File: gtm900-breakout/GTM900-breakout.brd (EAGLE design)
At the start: 70 x 70 mm, 110 parts, among them IC1 NCP303, IC2 CP2102N_28, J1 AUDIO-JACK3, K1 PJ-002BH-SMT-TR, T2 BC847, T3 BC847, U1 FH12A-40S-0.5SH(55), U2 MCP1827T-ADJE/ET, U3 MIC5366, U5 IP4234CZ6, U6 SN74AVC4T245-VQFN, X4 MINI-USB-SHIELD-UX60-MB-5ST, X5 OsmoSer

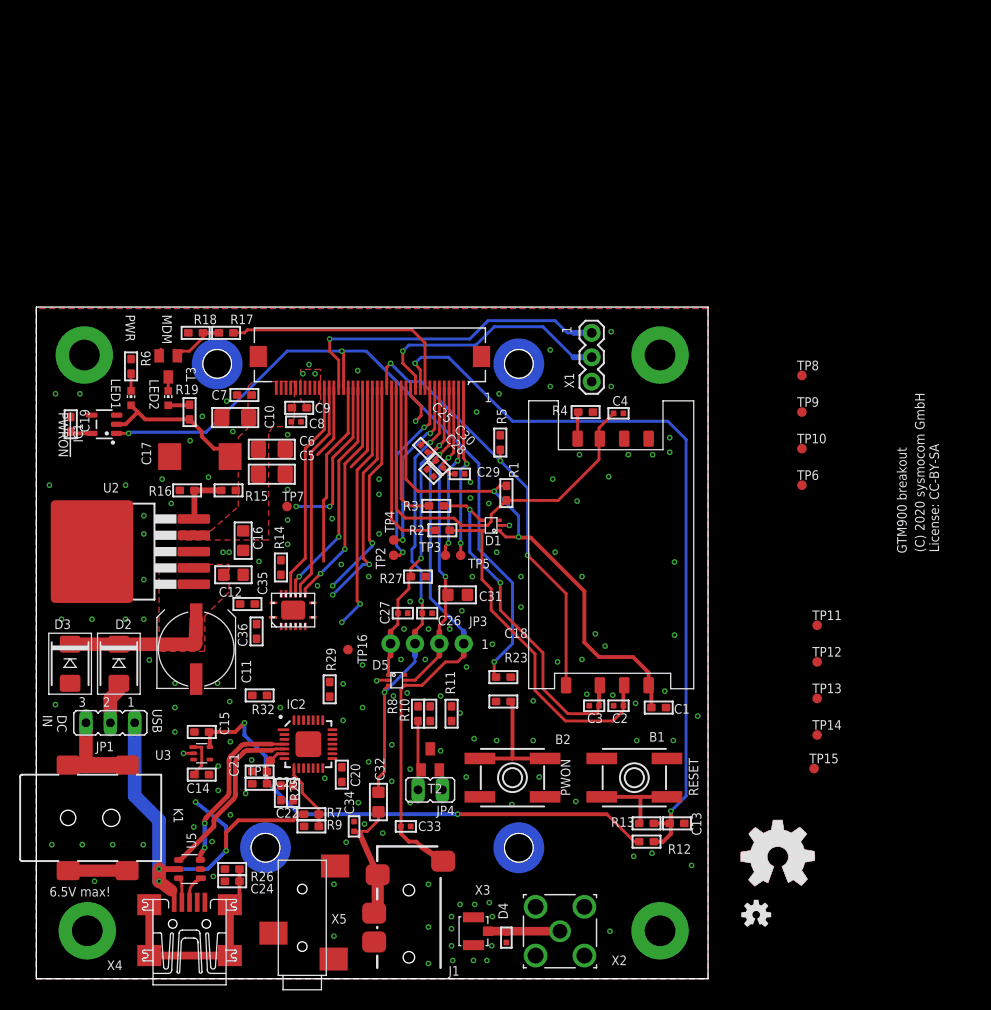
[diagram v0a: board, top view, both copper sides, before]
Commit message: gtm900-bo: rename main files w/o explicit version
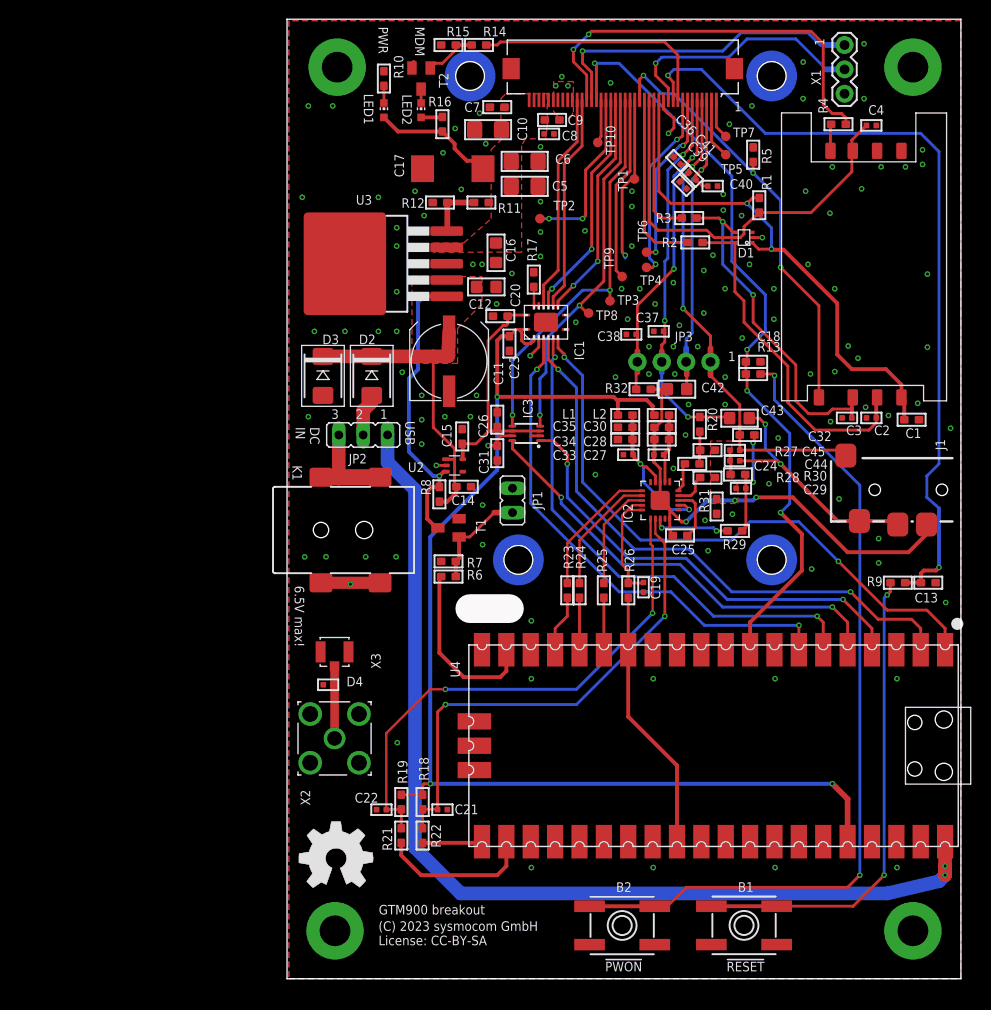
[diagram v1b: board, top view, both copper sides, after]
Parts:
- removed D5: PESD5V0UBV, laforge:SOT666
- removed JP4: (no value), jumper:JP1
- removed T3: BC847, transistor:SOT23-BEC
- removed TP11, TP12, TP13, TP14, TP15, TP16: TPTP10R, testpad:TP10R
- removed U$1: (no value), SparkFun-Aesthetics:OSHW-LOGO-S
- removed U5: IP4234CZ6, laforge:TSOP-6
- removed U6: SN74AVC4T245-VQFN, laforge:VQFN-N16
- removed X4: MINI-USB-SHIELD-UX60-MB-5ST, con-hirose:UX60-MB-5ST
- removed X5: OsmoSer, laforge:JACK2.5_SJ-2523
- added C37, C38, C39, C40, C41, C44, C45: 33p, rc-sysmocom:_0402
- added C42, C43: 10u, rc-sysmocom:_0805
- added IC3: TXB0102, TXB0102:VSSOP-8
- added JP2: (no value), jumper:JP2
- added L1, L2: 47nH, rc-sysmocom:_0603
- added R20: 22k, rc-sysmocom:_0603
- added R21, R22, R24: 220, rc-sysmocom:_0603
- added R28, R30: 1k, rc-sysmocom:_0603
- added R31: 0, rc-sysmocom:_0603
- added T1: BC847, transistor:SOT23-BEC
- added U4: RASPBERRY_PICOSMD, RpiPico:PICO-PKG-SMD
- C19: value 1u -> 33p; device rc-sysmocom:_0603 -> rc-sysmocom:_0402
- C20: value 1u -> 100n
- C21, C22, C36: value 100n -> 33p; device rc-sysmocom:_0603 -> rc-sysmocom:_0402
- C23: value 4.7u -> 100n
- C25, C30: value 33p -> 4.7u; device rc-sysmocom:_0402 -> rc-sysmocom:_0603
- C26, C28, C34: value 33p -> 100n; device rc-sysmocom:_0402 -> rc-sysmocom:_0603
- C31, C32: value 10u -> 100n; device rc-sysmocom:_0805 -> rc-sysmocom:_0603
- C35: value 100n -> 4.7u
- IC1: value NCP303 -> SN74AVC4T245-VQFN; device NCP303:SOT23-5 -> laforge:VQFN-N16
- IC2: value CP2102N_28 -> NAU88C10; device silabs_CP2102X:QFN28 -> NAU8810:QFN20
- JP1: device jumper:JP2 -> jumper:JP1
- R10, R16: value 22k -> 330
- R11: value 4.7k -> 200k
- R12: value DNP -> 22k
- R14: value 0 -> 22k
- R15: value 200k -> 22k
- R17: value 22k -> 0
- R18: value 22k -> 4,7k
- R19: value 330 -> 4,7k
- R23: value 1k -> 220
- R25: value 0 -> 220
- R26: value 1M -> 220
- R27: value 0 -> 1k
- R29: value 4K7 -> 22k
- R32: value 10k -> 0
- R6: value 330 -> 22k
- R8: value 22k -> 4.7k
- R9: value 47k -> 1k
- U2: value MCP1827T-ADJE/ET -> MIC5366; device ldo:TI_KTT_DPAK2 -> ldo:SC70-5
- U3: value MIC5366 -> MCP1827T-ADJE/ET; device ldo:SC70-5 -> ldo:TI_KTT_DPAK2
- moved J1 76.1 mm to (69.8, 51.0), turned to 180 degrees
- moved TP1 71.5 mm to (36.2, 83.3)
- moved T2 71.0 mm to (14.0, 93.8), turned to 180 degrees
- moved R12 70.0 mm to (15.9, 80.9), turned to 180 degrees
- moved R10 66.4 mm to (10.1, 93.8), turned to 270 degrees
- moved R9 66.2 mm to (63.7, 41.3), turned to 180 degrees
- moved C36 65.8 mm to (40.6, 85.2), turned to 135 degrees
- moved C24 64.7 mm to (42.2, 53.7)
- moved C19 62.1 mm to (37.1, 40.8)
- moved TP7 59.8 mm to (45.7, 87.8), turned to 180 degrees
- moved R14 58.2 mm to (20.0, 97.3), turned to 180 degrees
- moved R18 54.3 mm to (14.1, 18.4), turned to 90 degrees
- moved C32 54.2 mm to (47.9, 56.7), turned to 0 degrees
- moved R11 53.4 mm to (20.3, 80.9), turned to 0 degrees
- moved U3 53.2 mm to (6.03, 74.5), turned to 90 degrees
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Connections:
- net GPIO3/WAKEUP renamed SPKOUT-
- removed net CP_DTR: IC2.28, R8.1
- removed net CP_VDD: C21.2, C23.2, C36.2, IC2.6, R29.1, R32.2, TP1.TP, U6.1, U6.2
- removed net EN_VCC: R11.1, T2.C, U2.1, U3.3
- removed net GPIO0/TXT: IC2.19
- removed net GPIO1/RXT: IC2.18
- removed net GPIO2/RS485: IC2.17
- removed net GPIO4: IC2.22
- removed net GPIO5: IC2.21
- removed net GPIO6: IC2.20
- removed net N$23: C19.2, IC1.5
- removed net N$29: IC2.8, R7.2, R9.2
- removed net N$32: IC2.1, TP14.TP
- removed net USB_D_N: IC2.5, U5.4
- removed net USB_D_P: IC2.4, U5.3
- removed net _USB_DN: U5.6, X4.2
- removed net _USB_DP: U5.1, X4.3
- new net !MODEM_LDO_ON: R6.1, U4.P$19
- new net AGND: C25.1, C27.2, C28.2, C29.2, C30.2, C42.2, C44.1, C45.2, IC2.15, IC2.3, IC2.EXP, J1.4, R27.2, R28.2, R30.2, R31.1, R32.1
- new net MICBIAS: IC2.1
- new net MODEM_LDO_ON: R8.1, T1.C, U2.3, U3.1
- new net N$24: C27.1, C28.1, C30.1, IC2.2, L2.2
- new net N$25: C21.1, IC2.12, R18.1, R22.1
- new net N$26: C22.1, IC2.11, R19.1, R21.1
- new net N$28: C25.2, IC2.18
- new net N$31: C24.1, IC2.20
- new net PCM_CLK_RP2: R26.2, U4.P$14, U4.P$29
- new net PCM_FRAME_RP2: R25.2, U4.P$15
- new net PCM_MISO_RP2: R23.2, U4.P$17
- new net PCM_MOSI_RP2: R24.2, U4.P$16
- new net SCL: R21.2, U4.P$22
- new net SDA: R22.2, U4.P$21
- new net SPKOUT+: IC2.14
- new net SWGND: U4.P$42
- new net VCC: C23.2, C31.2, IC1.1, IC1.2, IC3.7, L1.1, L2.1, R18.2, R19.2, U4.P$36
- new net VSYS: U4.P$39
- new net _RXD2: IC1.4, U4.P$7
- new net _TXD2: IC1.6, U4.P$6
- new net _UART_CTS: IC3.1, U4.P$4
- new net _UART_RTS: IC3.8, U4.P$5
- net !PWON: now also R13.1, U4.P$9; no longer IC1.1, R23.1
- net !RST: now also R9.1; no longer R12.2, R13.1
- net AUXI+: now also TP5.TP; no longer TP3.TP
- net AUXI-: now also TP7.TP; no longer TP5.TP
- net AUXO+: now also TP4.TP; no longer TP2.TP
- net AUXO-: now also TP6.TP; no longer TP4.TP
- net EAR+: now also C36.2, C37.1, C43.2, R20.1; no longer C25.2, C26.1, C32.2, D5.3
- net EAR-: now also C36.1, C38.2, R32.2; no longer C25.1, C27.2, D5.1, R27.2
- net GND: now also C19.2, C20.2, C21.2, C22.2, C31.1, C34.2, C37.2, C38.1, C39.2, C40.2, IC1.8, IC1.9, IC2.5, IC3.2, JP1.2, R10.1, R12.2, R15.2, R17.2, R31.2, R7.2, T1.E, U2.2, U3.3, U3.PAD, U4.P$13, U4.P$18, U4.P$23, U4.P$28, U4.P$3, U4.P$33, U4.P$38, U4.P$8; no longer C19.1, C20.1, C21.1, C22.1, C24.1, C27.1, C28.2, C29.2, C31.2, C34.1, C36.1, D5.2, IC2.3, IC2.EXP, J1.4, JP4.2, R10.2, R14.2, R16.2, R18.2, R26.1, R27.1, R6.1, R9.1, T3.E, U2.3, U2.PAD, U3.2, U5.2, U6.3, U6.8, U6.9, X4.5, X5.1
- net LDO_IN: now also R8.2, U2.1, U3.2; no longer C20.2, C22.2, R11.2, R25.2, U2.2, U3.1
- net LPG: now also R14.1; no longer R17.1
- net MIC+: now also C32.1, C39.1, C41.1, C45.1; no longer C28.1, C30.1, C33.1, D5.4
- net MIC-: now also C40.1, C41.2, C42.1; no longer C29.1, C30.2, C31.1, D5.5
- net N$1: now also R10.2; no longer R6.2
- net N$11: now also C19.1, IC2.10, IC2.9, R26.1; no longer C24.2, R26.2, X4.M1, X4.M2, X4.M3, X4.M4
- net N$12: now also IC2.8, R25.1; no longer IC2.9, R29.2
- net N$14: now also IC2.7, R24.1; no longer IC2.2, TP13.TP
- net N$15: now also IC2.6, R23.1; no longer IC2.23, TP12.TP
- net N$16: now also C29.1, C32.2, R29.2, R30.1; no longer IC2.24, TP11.TP
- net N$17: now also JP1.1, R6.2, R7.1, T1.B; no longer IC2.7, R25.1
- net N$18: now also IC2.19, R28.1; no longer U6.6, X5.3
- net N$19: now also JP2.2; no longer JP1.2
- net N$2: now also R16.2; no longer R19.2
- net N$20: now also C33.1, C34.1, C35.1, IC2.17, IC2.4, L1.2; no longer R32.1, U6.4, X5.2
- net N$21: now also R9.2; no longer R13.2
- net N$22: now also IC1.14, IC1.15, R17.1; no longer R14.1, U6.14, U6.15
- net N$3: now also T2.C; no longer T3.C
- net N$30: now also IC2.13, R29.1; no longer IC2.27, TP15.TP
- net N$4: now also JP2.3; no longer JP1.3
- net N$5: now also R14.2, R15.1, T2.B; no longer R17.2, R18.1, T3.B
- net N$6: now also R11.1, R12.1, U3.5; no longer R15.1, R16.1, U2.5
- net N$7: now also C24.2, R20.2, R27.1; no longer JP4.1, R10.1, R8.2, T2.B
- net N$8: now also C43.1, C44.2; no longer C32.1, C34.2
- net N$9: now also R13.2; no longer R23.2
- net RXD2: now also IC1.13; no longer U6.13
- net TXD2: now also IC1.11; no longer U6.11
- net UART_CTS: now also IC3.4, TP8.TP; no longer TP10.TP
- net UART_DCD: now also TP1.TP; no longer TP6.TP
- net UART_DSR: now also TP10.TP; no longer TP9.TP
- net UART_DTR: now also TP9.TP; no longer TP16.TP
- net UART_RI: now also TP2.TP; no longer TP7.TP
- net UART_RTS: now also IC3.5, TP3.TP; no longer TP8.TP
- net UART_RXD: now also IC1.12; no longer U6.12
- net UART_TXD: now also IC1.10; no longer U6.10
- net USB_VBUS: now also JP2.1, U4.P$40; no longer JP1.1, R7.1, U5.5, X4.1
- net VCC_4V1: now also R11.2, R16.1, U3.4; no longer IC1.2, R15.2, R19.1, U2.4
- net VIO_2V8: now also C20.1, C26.1, IC1.16, IC3.3, IC3.6, U2.5; no longer C35.1, R12.1, U3.5, U6.16
- net _UART_RXD: now also IC1.5, U4.P$2; no longer IC2.25, U6.5
- net _UART_TXD: now also IC1.7, U4.P$1; no longer IC2.26, U6.7
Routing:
- net VCC: track 0.00 -> 131.9 mm, vias 0 -> 4
- net N$9: track 12.8 -> 86.8 mm, vias 0 -> 2
- net _UART_TXD: track 0.00 -> 63.9 mm, vias 0 -> 2
- net _UART_RXD: track 0.00 -> 61.2 mm, vias 0 -> 2
- net USB_VBUS: track 49.0 -> 107.2 mm, vias 4 -> 2
- net N$26: track 0.00 -> 54.4 mm, vias 0 -> 2
- net AGND: track 0.00 -> 54.3 mm, vias 0 -> 3
- net _TXD2: track 0.00 -> 54.0 mm, vias 0 -> 2
- net _RXD2: track 0.00 -> 53.5 mm, vias 0 -> 2
- net N$25: track 0.00 -> 52.1 mm, vias 0 -> 2
- net _UART_CTS: track 0.00 -> 47.5 mm, vias 0 -> 2
- net _UART_RTS: track 0.00 -> 46.5 mm, vias 0 -> 2
- net N$21: track 9.62 -> 50.1 mm, vias 0 -> 2
- net VDD: track 7.69 -> 43.3 mm, vias 0 -> 2
- net MODEM_LDO_ON: track 0.00 -> 31.3 mm, vias 0 -> 2
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- added copper zone on layer 1, net AGND
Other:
- board size 70 x 70 mm -> 70.2 x 100 mm
- board text added: "!PWON"
- board text added: "!RESET"
- board text added: "(C) 2023 sysmocom GmbH License: CC-BY-SA"
- board text removed: "!PWRON"
- board text removed: "(C) 2020 sysmocom GmbH License: CC-BY-SA"
- board text removed: "PWON"
- board text removed: "RESET"
